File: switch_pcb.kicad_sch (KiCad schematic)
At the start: 6 parts, among them J1 3x5mm, SW1 Microswitch

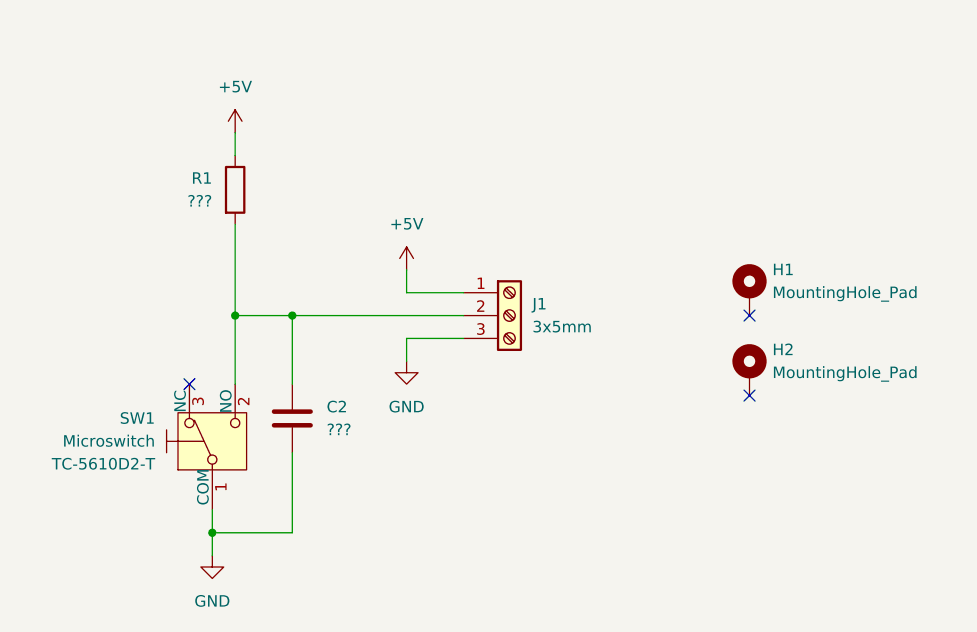
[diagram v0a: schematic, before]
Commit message: Switch back to the previous circuit with switch at the top
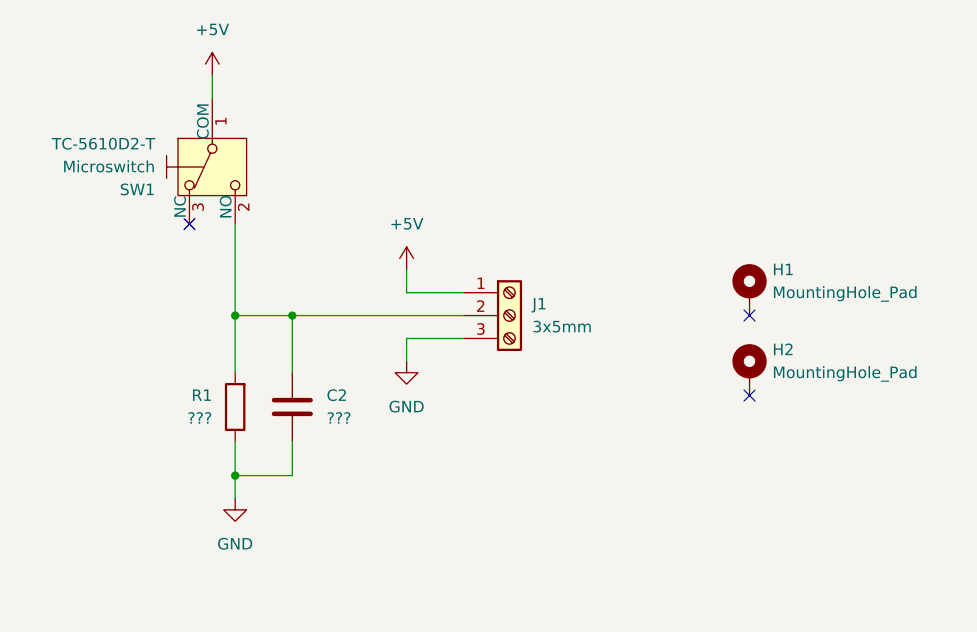
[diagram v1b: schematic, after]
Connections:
- net +5V: now also SW1.1 (COM); no longer R1.1
- net GND: now also R1.1; no longer SW1.1 (COM)
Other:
- moved on the sheet: C2, R1, SW1
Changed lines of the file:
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@@
 	)
 	(junction
-		(at 114.3 109.22)
+		(at 116.84 102.87)
 		(diameter 0)
 		(color 0 0 0 0)
@@
 	)
 	(no_connect
-		(at 111.76 92.71)
+		(at 111.76 74.93)
 	)
 	(no_connect
@@
 	(wire
 		(pts
-			(xy 114.3 106.68) (xy 114.3 109.22)
+			(xy 116.84 99.06) (xy 116.84 102.87)
 		)
 		(stroke
@@
 	(wire
 		(pts
-			(xy 123.19 85.09) (xy 123.19 92.71)
+			(xy 123.19 85.09) (xy 123.19 91.44)
 		)
 		(stroke
@@
 	(wire
 		(pts
-			(xy 123.19 100.33) (xy 123.19 109.22)
-		)
-		(stroke
-			(width 0)
-			(type default)
-		)
-	)
-	(wire
-		(pts
-			(xy 114.3 109.22) (xy 114.3 111.76)
-		)
-		(stroke
-			(width 0)
-			(type default)
-		)
-	)
-	(wire
-		(pts
-			(xy 116.84 64.77) (xy 116.84 67.31)
+			(xy 123.19 99.06) (xy 123.19 102.87)
+		)
+		(stroke
+			(width 0)
+			(type default)
+		)
+	)
+	(wire
+		(pts
+			(xy 116.84 102.87) (xy 116.84 105.41)
+		)
+		(stroke
+			(width 0)
+			(type default)
+		)
+	)
+	(wire
+		(pts
+			(xy 114.3 58.42) (xy 114.3 60.96)
 		)
 		(stroke
@@
 	(wire
 		(pts
-			(xy 116.84 92.71) (xy 116.84 85.09)
-		)
-		(stroke
-			(width 0)
-			(type default)
-		)
-	)
-	(wire
-		(pts
-			(xy 114.3 109.22) (xy 123.19 109.22)
+			(xy 116.84 91.44) (xy 116.84 85.09)
+		)
+		(stroke
+			(width 0)
+			(type default)
+		)
+	)
+	(wire
+		(pts
+			(xy 116.84 102.87) (xy 123.19 102.87)
 		)
 		(stroke
@@
 	(symbol
 		(lib_id "power:GND")
-		(at 114.3 111.76 0)
+		(at 116.84 105.41 0)
 		(unit 1)
 		(exclude_from_sim no)
@@
 		(fields_autoplaced yes)
 		(property "Reference" "#PWR06"
-			(at 114.3 118.11 0)
+			(at 116.84 111.76 0)
 			(effects
 				(font
@@
 		)
 		(property "Value" "GND"
-			(at 114.3 116.84 0)
+			(at 116.84 110.49 0)
 			(effects
 				(font
@@
 		)
 		(property "Footprint" ""
-			(at 114.3 111.76 0)
+			(at 116.84 105.41 0)
 			(effects
 				(font
@@
 		)
 		(property "Datasheet" ""
-			(at 114.3 111.76 0)
+			(at 116.84 105.41 0)
 			(effects
 				(font
@@
 		)
 		(property "Description" "Power symbol creates a global label with name \"GND\" , ground"
-			(at 114.3 111.76 0)
+			(at 116.84 105.41 0)
 			(effects
 				(font
@@
 	(symbol
 		(lib_id "Device:R")
-		(at 116.84 71.12 0)
+		(at 116.84 95.25 180)
 		(unit 1)
 		(exclude_from_sim no)
@@
 		(fields_autoplaced yes)
 		(property "Reference" "R1"
-			(at 114.3 69.8499 0)
-			(effects
-				(font
-					(size 1.27 1.27)
-				)
-				(justify right)
+			(at 114.3 93.9799 0)
+			(effects
+				(font
+					(size 1.27 1.27)
+				)
+				(justify left)
 			)
 		)
 		(property "Value" "???"
-			(at 114.3 72.3899 0)
-			(effects
-				(font
-					(size 1.27 1.27)
-				)
-				(justify right)
+			(at 114.3 96.5199 0)
+			(effects
+				(font
+					(size 1.27 1.27)
+				)
+				(justify left)
 			)
 		)
 		(property "Footprint" "Resistor_THT:R_Axial_DIN0207_L6.3mm_D2.5mm_P10.16mm_Horizontal"
-			(at 115.062 71.12 90)
+			(at 118.618 95.25 90)
 			(effects
 				(font
@@
 		)
 		(property "Datasheet" "~"
-			(at 116.84 71.12 0)
+			(at 116.84 95.25 0)
 			(effects
 				(font
@@
 		)
 		(property "Description" "Resistor"
-			(at 116.84 71.12 0)
+			(at 116.84 95.25 0)
 			(effects
 				(font
@@
 	(symbol
 		(lib_id "power:+5V")
-		(at 116.84 64.77 0)
+		(at 114.3 58.42 0)
 		(unit 1)
 		(exclude_from_sim no)
@@
 		(fields_autoplaced yes)
 		(property "Reference" "#PWR03"
-			(at 116.84 68.58 0)
+			(at 114.3 62.23 0)
 			(effects
 				(font
@@
 		)
 		(property "Value" "+5V"
-			(at 116.84 59.69 0)
+			(at 114.3 53.34 0)
 			(effects
 				(font
@@
 		)
 		(property "Footprint" ""
-			(at 116.84 64.77 0)
+			(at 114.3 58.42 0)
 			(effects
 				(font
@@
 		)
 		(property "Datasheet" ""
-			(at 116.84 64.77 0)
+			(at 114.3 58.42 0)
 			(effects
 				(font
@@
 		)
 		(property "Description" "Power symbol creates a global label with name \"+5V\""
-			(at 116.84 64.77 0)
+			(at 114.3 58.42 0)
 			(effects
 				(font
@@
 	(symbol
 		(lib_id "microswitch:SW_Push_SPDT")
-		(at 114.3 99.06 90)
+		(at 114.3 68.58 90)
+		(mirror x)
 		(unit 1)
 		(exclude_from_sim no)
@@
 		(dnp no)
 		(property "Reference" "SW1"
-			(at 107.95 96.5199 90)
+			(at 107.95 71.1201 90)
 			(effects
 				(font
@@
 		)
 		(property "Value" "Microswitch"
-			(at 107.95 99.0599 90)
+			(at 107.95 68.5801 90)
 			(effects
 				(font
@@
 		)
 		(property "Footprint" "switch_pcb:TC-5610D2-T"
-			(at 114.3 99.06 0)
+			(at 114.3 68.58 0)
 			(effects
 				(font
@@
 		)
 		(property "Datasheet" "https://www.lcsc.com/datasheet/lcsc_datasheet_2004101009_Yuandi-TC-5610D2-T_C504864.pdf"
-			(at 114.3 99.06 0)
+			(at 114.3 68.58 0)
 			(effects
 				(font
@@
 		)
 		(property "Description" "Momentary Switch, single pole double throw"
-			(at 105.41 99.06 0)
+			(at 105.41 68.58 0)
 			(effects
 				(font
@@
 		)
 		(property "JLC" "C504864"
-			(at 114.3 99.06 90)
+			(at 114.3 68.58 90)
 			(effects
 				(font
@@
 		)
 		(property "MFR" "TC-5610D2-T "
-			(at 107.95 101.5999 90)
+			(at 107.95 66.0401 90)
 			(effects
 				(font
@@
 	(symbol
 		(lib_id "Device:C")
-		(at 123.19 96.52 0)
+		(at 123.19 95.25 0)
 		(unit 1)
 		(exclude_from_sim no)
@@
 		(fields_autoplaced yes)
 		(property "Reference" "C2"
-			(at 127 95.2499 0)
+			(at 127 93.9799 0)
 			(effects
 				(font
@@
 		)
 		(property "Value" "???"
-			(at 127 97.7899 0)
+			(at 127 96.5199 0)
 			(effects
 				(font
@@
 		)
 		(property "Footprint" "Capacitor_THT:C_Disc_D9.0mm_W5.0mm_P5.00mm"
-			(at 124.1552 100.33 0)
+			(at 124.1552 99.06 0)
 			(effects
 				(font
@@
 		)
 		(property "Datasheet" "~"
-			(at 123.19 96.52 0)
+			(at 123.19 95.25 0)
 			(effects
 				(font
@@
 		)
 		(property "Description" "Unpolarized capacitor"
-			(at 123.19 96.52 0)
-			(effects
-				(font
+			(at 123.19 95.25 0)
+			(effects
+				(font
